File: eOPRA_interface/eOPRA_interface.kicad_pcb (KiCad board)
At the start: 4 copper layers, 76 x 57.9 mm, 182 parts, among them J1 CONN_01X04_MALE, J2 CONN_01X04_MALE, J3 CONN_01X04_MALE, J4 CONN_01X02_MALE, J5 CONN_01X04_MALE, J6 CONN_02X10, J8 CONN_01X04_MALE, Q1 G3VM-351VY1-TR05, Q10 Q_NMOS_GSD, Q11 G3VM-351VY1-TR05, Q12 Q_NMOS_GSD, Q13 Q_NMOS_GSD, Q14 G3VM-351VY1-TR05, Q15 G3VM-351VY1-TR05, Q16 Q_NMOS_GSD, Q17 G3VM-351VY1-TR05, Q18 G3VM-351VY1-TR05, Q19 Q_NMOS_GSD, Q2 Q_NMOS_GSD, Q20 G3VM-351VY1-TR05, Q21 Q_NMOS_GSD, Q22 G3VM-351VY1-TR05, Q23 G3VM-351VY1-TR05, Q24 Q_NMOS_GSD, Q25 Q_NMOS_GSD, Q26 G3VM-351VY1-TR05, Q27 G3VM-351VY1-TR05, Q28 Q_NMOS_GSD, Q29 Q_NMOS_GSD, Q3 Q_NMOS_GSD, Q30 G3VM-351VY1-TR05, Q31 G3VM-351VY1-TR05, Q32 Q_NMOS_GSD, Q33 Q_NMOS_GSD, Q34 G3VM-351VY1-TR05, Q4 Q_NMOS_GSD, Q5 Q_PMOS_GSD, Q6 Q_NMOS_GSD, Q7 G3VM-351VY1-TR05, Q8 Q_NMOS_GSD, Q9 G3VM-351VY1-TR05, SW2 SW_Push, SW3 SW_Push, SW4 SW_SPST, SW6 SW_Push, SW7 Rotary_Encoder_Switch, U1 USB_C_2.0, U10 RP2040, U11 W25Q128JVS, U13 MCP25625, U14 AP2205-50, U15 AP2213-8_SOIC, U17 74HC238, U2 ARM-SWD-10, U3 AP2213-8_SOIC, U4 DS3231MZ+, U5 XT-X, U6 Mounting-holes, U7 Mounting-holes, U8 Mounting-holes, U9 Mounting-holes, Y1 16Mhz 12pF, Y3 12Mhz 12pF

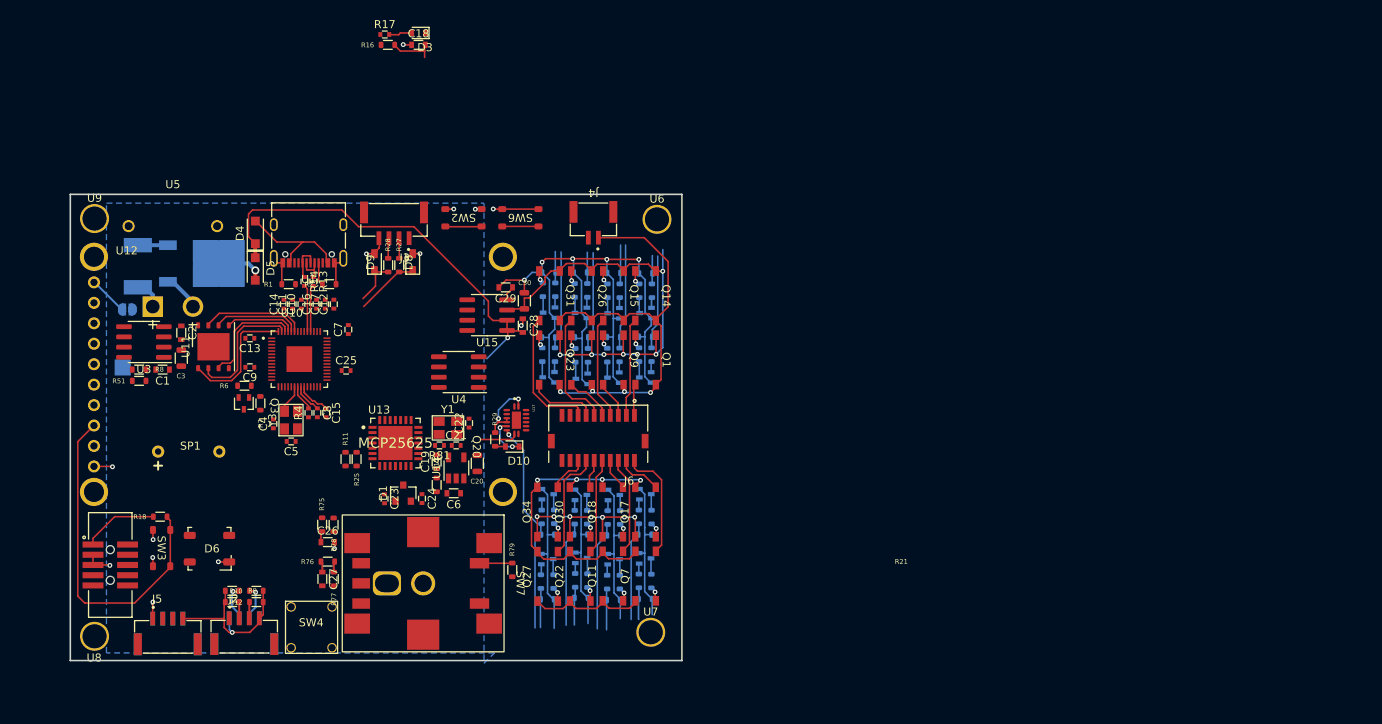
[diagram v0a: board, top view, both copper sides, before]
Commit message: preliminary finish
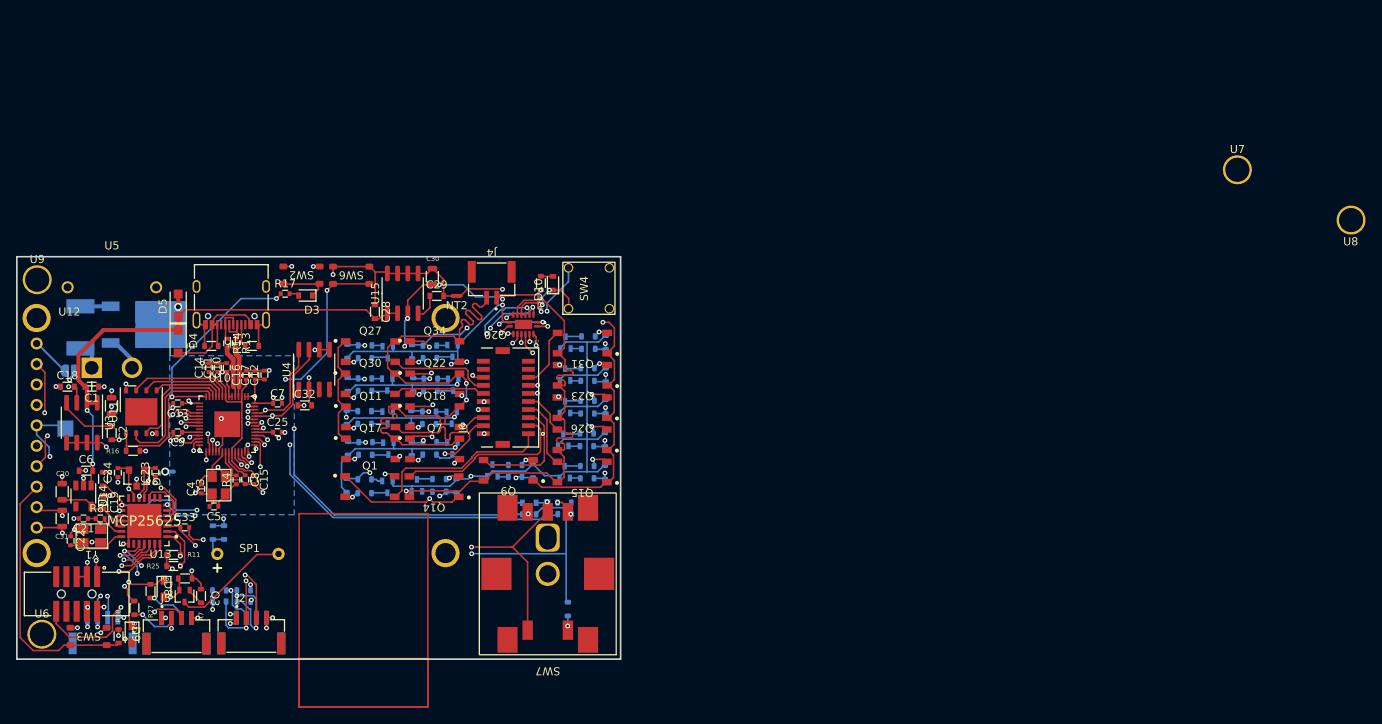
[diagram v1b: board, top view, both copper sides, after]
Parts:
- removed D6: WS2812B, 1_Semi_LED-Opto:WS2812B
- added C31: 10u, 2_Passives_Capacitors_SMD_IPC:C_2012_805_B, F.Cu at (105.6, 107.5)
- added C32: 0.1u, 2_Passives_Capacitors_SMD_IPC:C_1608_603_B, F.Cu at (135.8, 93.5)
- added C33: 1uF, 2_Passives_Resistors_SMD_IPC:R_1005_402_A, F.Cu at (120.8, 108.6)
- added NT1: net-tie, 0_NetTie:NetTie-2_SMD_Pad0.5mm, B.Cu at (119.0, 101.7)
- added NT2: net-tie, 0_NetTie:NetTie-2_SMD_Pad0.5mm, F.Cu at (154.6, 79.9)
- C26, C27, J3, R10, R12, R21, R51, R75, R76, R77, R78, R79, R8, R9: moved to B.Cu
- moved U8 164.4 mm to (265.8, 70.5)
- moved U7 92.8 mm to (251.6, 64.2)
- moved U6 92.2 mm to (103.1, 121.9)
- moved C18 60.9 mm to (106.3, 91.2)
- moved R16 59.6 mm to (114.4, 99.1)
- moved J3 58.4 mm to (119.8, 122.2)
- moved D9 55.1 mm to (114.3, 121.9), turned to -90 degrees
- moved SW4 54.4 mm to (171.0, 79.0), turned to 90 degrees
- moved R28 53.0 mm to (114.6, 118.6), turned to 90 degrees
- moved C20 51.7 mm to (105.6, 104.2), turned to -90 degrees
- moved C22 51.6 mm to (106.7, 110.3), turned to -90 degrees
- moved D8 50.9 mm to (118.3, 116.2), turned to -90 degrees
- moved R27 50.9 mm to (116.6, 116.5), turned to 90 degrees
- moved C21 47.2 mm to (108.3, 107.5), turned to 180 degrees
- moved U14 46.4 mm to (108.3, 104.7), turned to -90 degrees
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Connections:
- C10 pad 2: GND -> GNDD
- C11 pad 2: GND -> GNDD
- C12 pad 2: GND -> GNDD
- C13 pad 2: GND -> GNDD
- C14 pad 2: GND -> GNDD
- C15 pad 2: GND -> GNDD
- C16 pad 2: GND -> GNDD
- C17 pad 2: GND -> GNDD
- C25 pad 2: GND -> GNDD
- C29 pad 2: GNDD -> GND
- C30 pad 1: GNDD -> GND
- C4 pad 1: GND -> GNDD
- C5 pad 2: GND -> GNDD
- C7 pad 2: GND -> GNDD
- C8 pad 2: GND -> GNDD
- C9 pad 2: GND -> GNDD
- Q10 pad 2: GNDD -> GNDREF
- Q12 pad 2: GNDD -> GNDREF
- Q13 pad 2: GNDD -> GNDREF
- Q16 pad 2: GNDD -> GNDREF
- Q19 pad 2: GNDD -> GNDREF
- Q2 pad 2: GNDD -> GNDREF
- Q21 pad 2: GNDD -> GNDREF
- Q24 pad 2: GNDD -> GNDREF
- Q25 pad 2: GNDD -> GNDREF
- Q28 pad 2: GNDD -> GNDREF
- Q29 pad 2: GNDD -> GNDREF
- Q32 pad 2: GNDD -> GNDREF
- Q33 pad 2: GNDD -> GNDREF
- Q4 pad 2: GNDD -> GNDREF
- Q6 pad 2: GNDD -> GNDREF
- Q8 pad 2: GNDD -> GNDREF
- R19 pad 1: GNDD -> GNDREF
- R3 pad 1: GNDD -> GNDREF
- R30 pad 1: GNDD -> GNDREF
- R33 pad 1: GNDD -> GNDREF
- R36 pad 1: GNDD -> GNDREF
- R39 pad 1: GNDD -> GNDREF
- R40 pad 1: GNDD -> GNDREF
- R45 pad 1: GNDD -> GNDREF
- R50 pad 1: GNDD -> GNDREF
- R52 pad 1: GNDD -> GNDREF
- R57 pad 1: GNDD -> GNDREF
- R58 pad 1: GNDD -> GNDREF
- R63 pad 1: GNDD -> GNDREF
- R64 pad 1: GNDD -> GNDREF
- R69 pad 1: GNDD -> GNDREF
- R70 pad 1: GNDD -> GNDREF
- SW4 pad 2: GND -> GNDREF
- U10 pad 19: GND -> GNDD
- U10 pad 57: GND -> GNDD
- U10 pad 9: /processor/LED_CTL -> unconnected-(U10-GPIO7-Pad9)
- U15 pad 7: GNDD -> GND
- U15 pad 8: GNDD -> GND
- U17 pad 17: unconnected-(U17-EP-Pad17) -> (no net)
- U17 pad 8: GND -> GNDREF
- Y3 pad 2: GND -> GNDD
- Y3 pad 4: GND -> GNDD
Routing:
- net GNDREF: track 0.00 -> 182.2 mm, vias 0 -> 8
- net GNDD: track 164.4 -> 23.5 mm, vias 5 -> 10
- net /~{RESET}: track 4.50 -> 72.7 mm, vias 0 -> 4
- net GND: track 42.0 -> 108.5 mm, vias 14 -> 37
- net /processor/ENC_CTL_0: track 0.00 -> 54.9 mm, vias 0 -> 3
- net /processor/ENC_CTL_1: track 0.00 -> 54.2 mm, vias 0 -> 3
- net /processor/ENC_CTL_2: track 0.00 -> 54.1 mm, vias 0 -> 3
- net +3V3: track 39.4 -> 91.8 mm, vias 1 -> 27
- net /ROT_ENC_0: track 1.20 -> 48.2 mm, vias 0 -> 2
- net /SCL1: track 2.01 -> 47.5 mm, vias 0 -> 3
- net /SDA1: track 1.83 -> 46.2 mm, vias 0 -> 3
- net /ROT_ENC_1: track 1.36 -> 44.4 mm, vias 0 -> 2
- net /switch_control/CHAN_2: track 18.2 -> 54.8 mm, vias 0 -> 3
- net /switch_control/CHAN_1: track 16.0 -> 50.9 mm, vias 0 -> 3
- net /processor/CAN_INT: track 0.00 -> 34.0 mm, vias 0 -> 3
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- added copper zone on In1.Cu, net +3V3
- added copper zone on In2.Cu, net GND
- added copper zone on B.Cu, net GNDD
- added copper zone on In2.Cu, net GNDREF
- added copper zone on In1.Cu, net SWITCHING_3V3
- removed copper zone on B.Cu, net GND
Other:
- board size 76 x 57.9 mm -> 75 x 50 mm
